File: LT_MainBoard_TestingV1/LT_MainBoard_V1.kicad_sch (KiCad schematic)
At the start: 24 parts, among them CN1 NUCLEO-L432KC, J1 Molar Nanofit Connectors, U1 ISO1050DUB, U2 MCP2515-I/SO, U3 XBP9B-DPST-001, U4 LM7809_TO220, U5 LM7805_TO220, U6 LF33_TO220

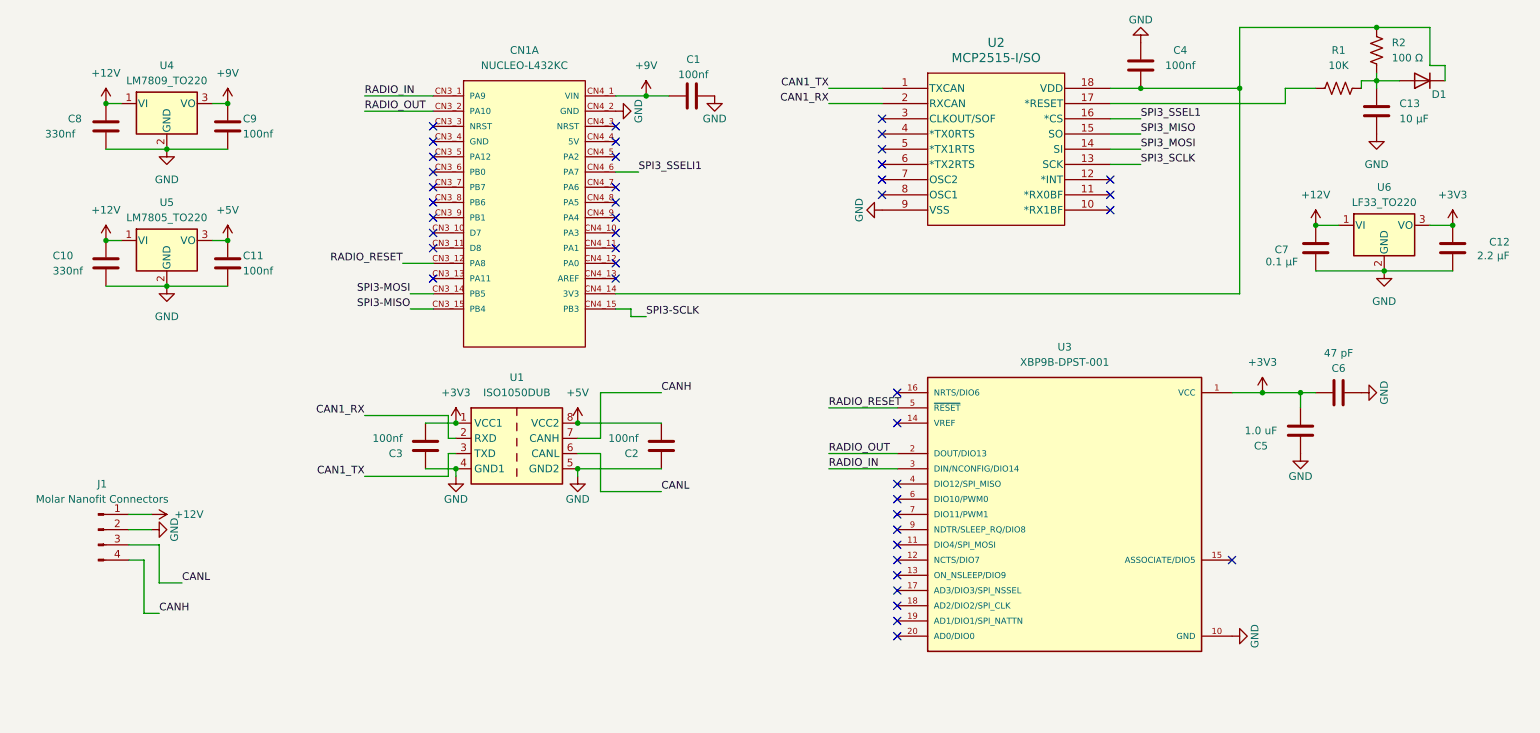
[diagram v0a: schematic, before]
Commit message: update LT board to F446RE
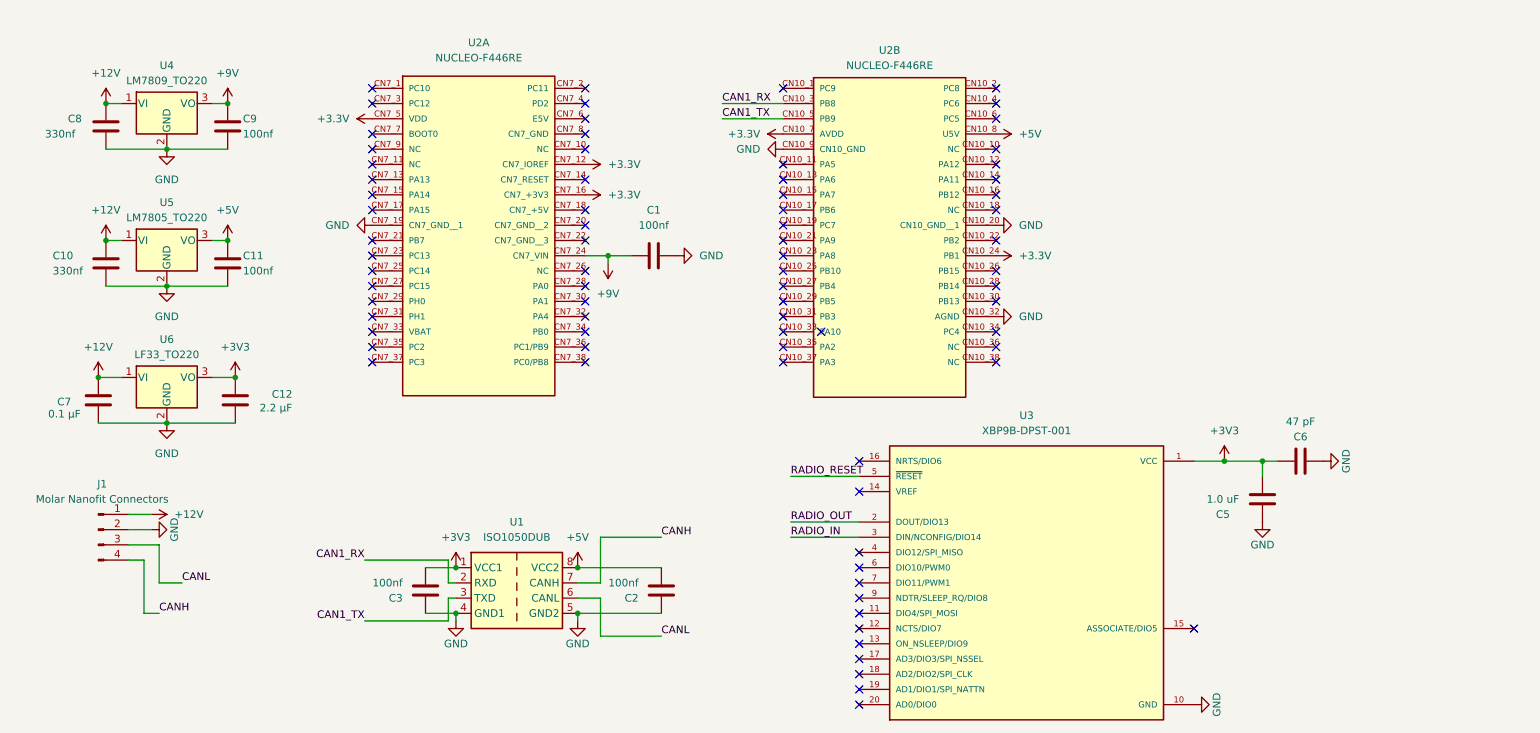
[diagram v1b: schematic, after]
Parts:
- removed C13: 10 µF, Capacitor_SMD:C_0805_2012Metric, symbol Device:C
- removed C4: 100nf, Capacitor_SMD:C_0805_2012Metric_Pad1.18x1.45mm_HandSolder, symbol Device:C
- removed CN1: NUCLEO-L432KC, FS_3_Global_Footprint_Library:NUCLEO-L432KC, symbol FS_3_Global_Symbol_Library:NUCLEO-L432KC
- removed D1: D, Diode_SMD:D_0805_2012Metric, symbol Device:D
- removed R1: 10K, Resistor_SMD:R_0805_2012Metric, symbol Device:R_US
- removed R2: 100 Ω, Resistor_SMD:R_0805_2012Metric, symbol Device:R_US
- removed U2: MCP2515-I/SO, Package_SO:SOIC-18W_7.5x11.6mm_P1.27mm, symbol FS_3_Global_Symbol_Library:MCP2515-I_SO
- added U2: NUCLEO-F446RE, FS_3_Global_Footprint_Library:NUCLEO-F446RE, symbol FS_3_Global_Symbol_Library:NUCLEO-F446RE
- C1: footprint Capacitor_SMD:C_0805_2012Metric_Pad1.18x1.45mm_HandSolder -> Capacitor_SMD:C_0805_2012Metric
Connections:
- net +5V: now also U2.CN10_8 (U5V)
- net +9V: now also U2.CN7_24 (CN7_VIN)
- net CAN1_RX: now also U2.CN10_3 (PB8)
- net CAN1_TX: now also U2.CN10_5 (PB9)
- net GND: now also U2.CN10_20 (CN10_GND__1), U2.CN10_32 (AGND), U2.CN10_9 (CN10_GND), U2.CN7_19 (CN7_GND__1)
- new net +3.3V: U2.CN10_24 (PB1), U2.CN10_7 (AVDD), U2.CN7_12 (CN7_IOREF), U2.CN7_16 (CN7_+3V3), U2.CN7_5 (VDD)
- no-connect marks 43 -> 78
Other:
- moved on the sheet: C12, C2, C3, C5, C6, C7, U1, U3, U6
